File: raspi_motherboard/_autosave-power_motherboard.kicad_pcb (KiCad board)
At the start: 4 copper layers, 65 x 59.9 mm, 62 parts, among them J1 GPIO, J2 Conn_02x04_Top_Bottom, J3 Conn_01x03, U1 MCP2515-xST, U2 SN65HVD230, U3 TPS563200, Y1 AMB8-12Mhz

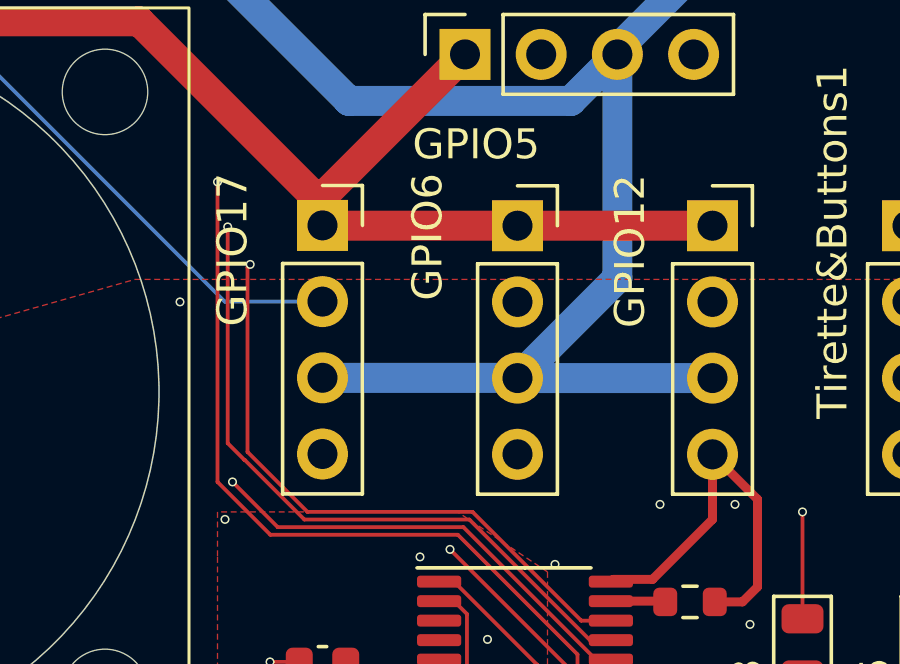
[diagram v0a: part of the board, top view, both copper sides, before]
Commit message: Last update
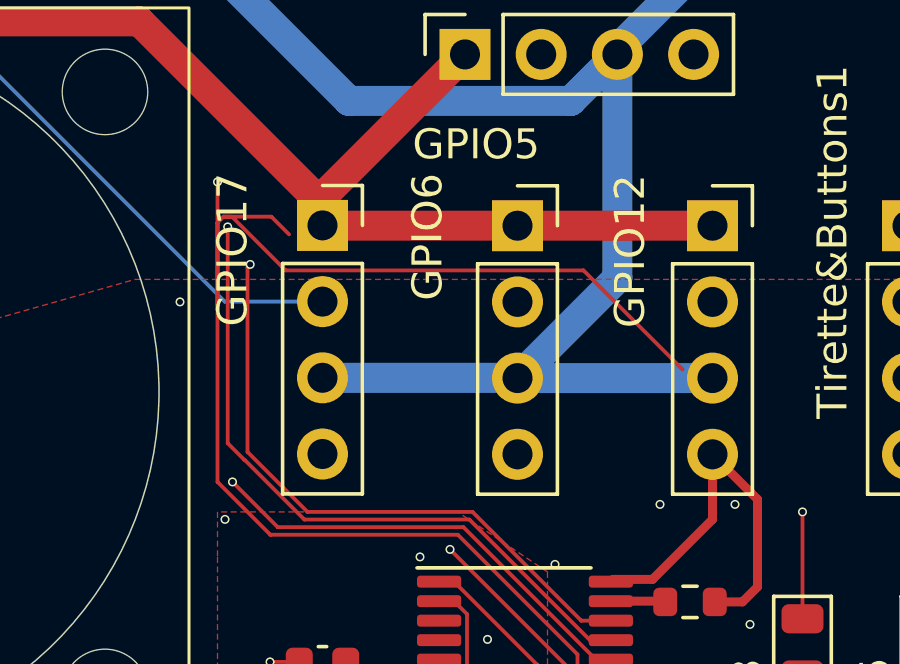
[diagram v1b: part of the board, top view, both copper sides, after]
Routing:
- net R_CLK: track 36.0 -> 59.0 mm
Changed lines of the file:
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@@
 		(tags "resistor")
 		(property "Reference" "R_12VE_1"
-			(at 0 1.43 360)
+			(at 0 1.43 0)
 			(layer "Dwgs.User")
 			(effects
@@
 		)
 		(property "Value" "10k"
-			(at 5.945 21.065 360)
+			(at 5.945 21.065 0)
 			(layer "B.Fab")
 			(effects
@@
 		)
 		(property "Footprint" "Resistor_SMD:R_0603_1608Metric"
-			(at 0 0 360)
+			(at 0 0 0)
 			(layer "F.Fab")
 			(hide yes)
@@
 		)
 		(property "Datasheet" ""
-			(at 0 0 360)
+			(at 0 0 0)
 			(layer "F.Fab")
 			(hide yes)
@@
 		)
 		(property "Description" ""
-			(at 0 0 360)
+			(at 0 0 0)
 			(layer "F.Fab")
 			(hide yes)
@@
 		)
 		(fp_text user "${REFERENCE}"
-			(at 0 0 360)
+			(at 0 0 0)
 			(layer "B.Fab")
 			(effects
@@
 	)
 	(segment
+		(start 140.23104 57.9095)
+		(end 142.02104 59.6995)
+		(width 0.127)
+		(layer "F.Cu")
+		(net 12)
+	)
+	(segment
 		(start 152.8625 73.975)
 		(end 152.364171 73.975)
@@
 	)
 	(segment
+		(start 139.94896 57.9095)
+		(end 141.546 57.9095)
+		(width 0.127)
+		(layer "F.Cu")
+		(net 12)
+	)
+	(segment
+		(start 139.75 61)
+		(end 139.75 56.75)
+		(width 0.127)
+		(layer "F.Cu")
+		(net 12)
+	)
+	(segment
+		(start 141.546 57.9095)
+		(end 142.1365 58.5)
+		(width 0.127)
+		(layer "F.Cu")
+		(net 12)
+	)
+	(segment
 		(start 152.364171 73.975)
 		(end 151.75 73.360829)
@@
 	(segment
 		(start 139.75 66.75)
-		(end 139.75 56.75)
+		(end 139.75 61)
+		(width 0.127)
+		(layer "F.Cu")
+		(net 12)
+	)
+	(segment
+		(start 139.94896 57.9095)
+		(end 140.23104 57.9095)
+		(width 0.127)
+		(layer "F.Cu")
+		(net 12)
+	)
+	(segment
+		(start 142.02104 59.6995)
+		(end 151.9495 59.6995)
+		(width 0.127)
+		(layer "F.Cu")
+		(net 12)
+	)
+	(segment
+		(start 139.75 61)
+		(end 139.75 58.10846)
 		(width 0.127)
 		(layer "F.Cu")
@@
 		(width 0.127)
 		(layer "F.Cu")
+		(net 12)
+	)
+	(segment
+		(start 139.75 58.10846)
+		(end 139.94896 57.9095)
+		(width 0.127)
+		(layer "F.Cu")
+		(net 12)
+	)
+	(segment
+		(start 151.9495 59.6995)
+		(end 155.25 63)
+		(width 0.127)
+		(layer "F.Cu")
